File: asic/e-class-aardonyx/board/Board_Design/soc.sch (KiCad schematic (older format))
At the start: 90 parts, among them J1 Conn_01x04, U1 SKT32E, U2 CDCE913PW, Y1 10MHz

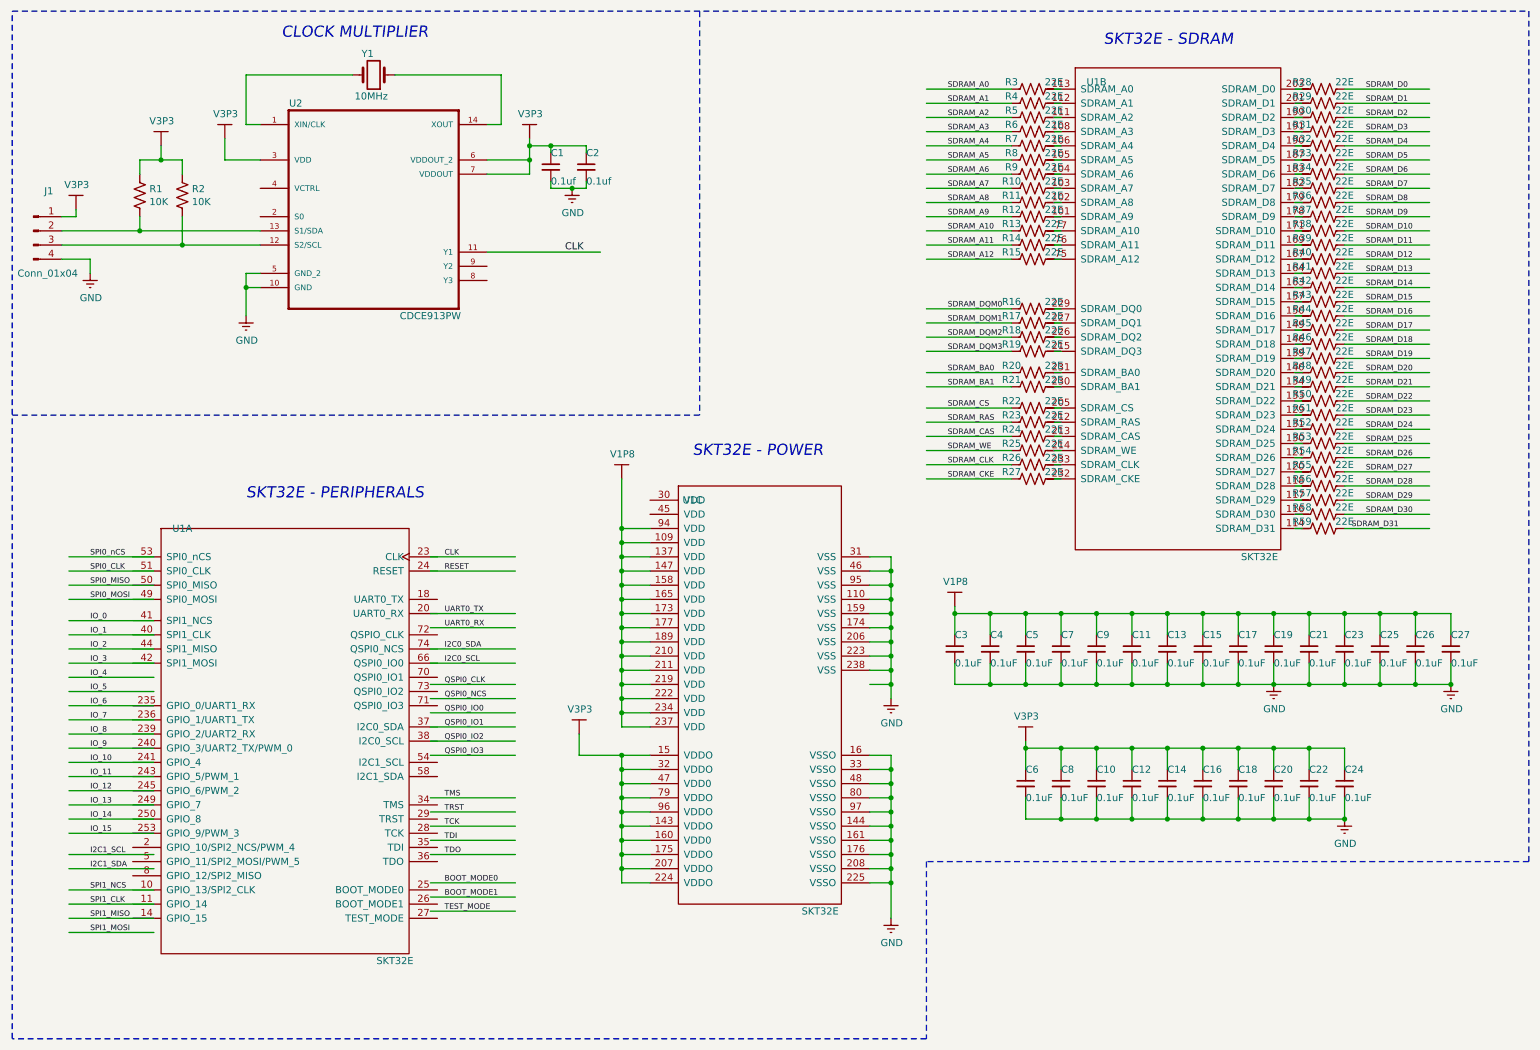
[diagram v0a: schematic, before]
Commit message: update
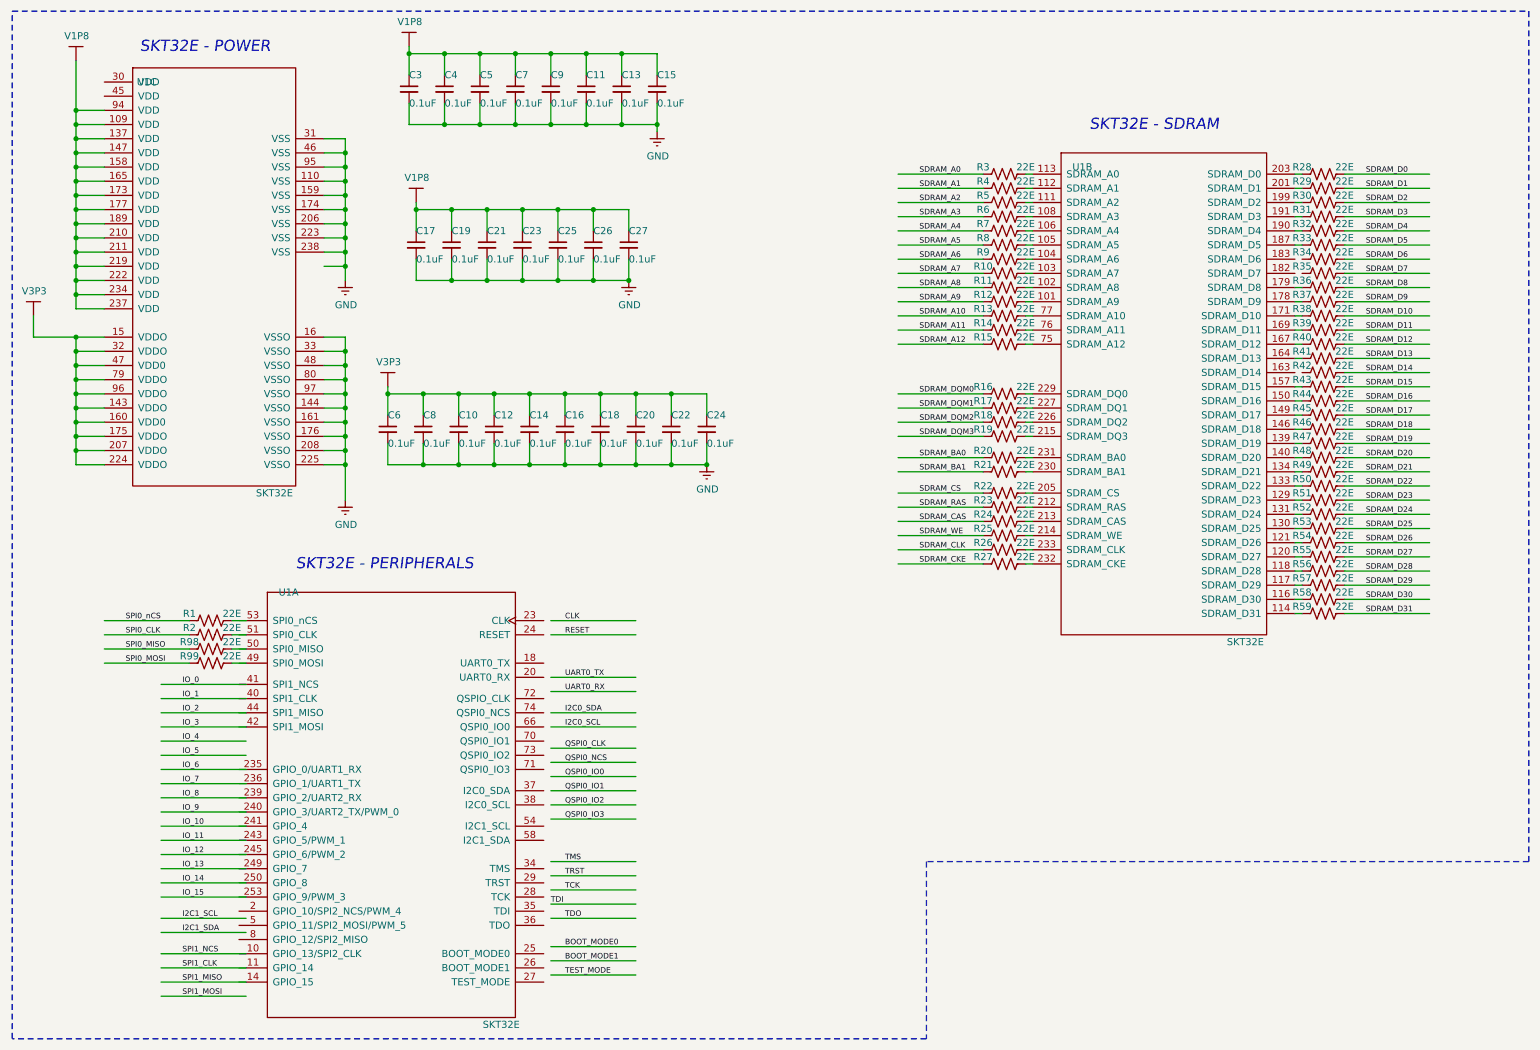
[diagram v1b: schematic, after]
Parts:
- removed C1, C2: 0.1uf, symbol aardonyx:C_Small
- removed J1: Conn_01x04, symbol Connector:Conn_01x04_Male
- removed U2: CDCE913PW, SOP65P640X120-14N, symbol aardonyx:CDCE913PW
- removed Y1: 10MHz, symbol aardonyx:Crystal
- added R98, R99: 22E, symbol aardonyx:R_US
- R1, R2: value 10K -> 22E
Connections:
- wire segments 390 -> 350
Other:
- note removed: "CLOCK MULTIPLIER\n"
- moved on the sheet: C10, C11, C12, C13, C14, C15, C16, C17, C18, C19, C20, C21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

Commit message: update
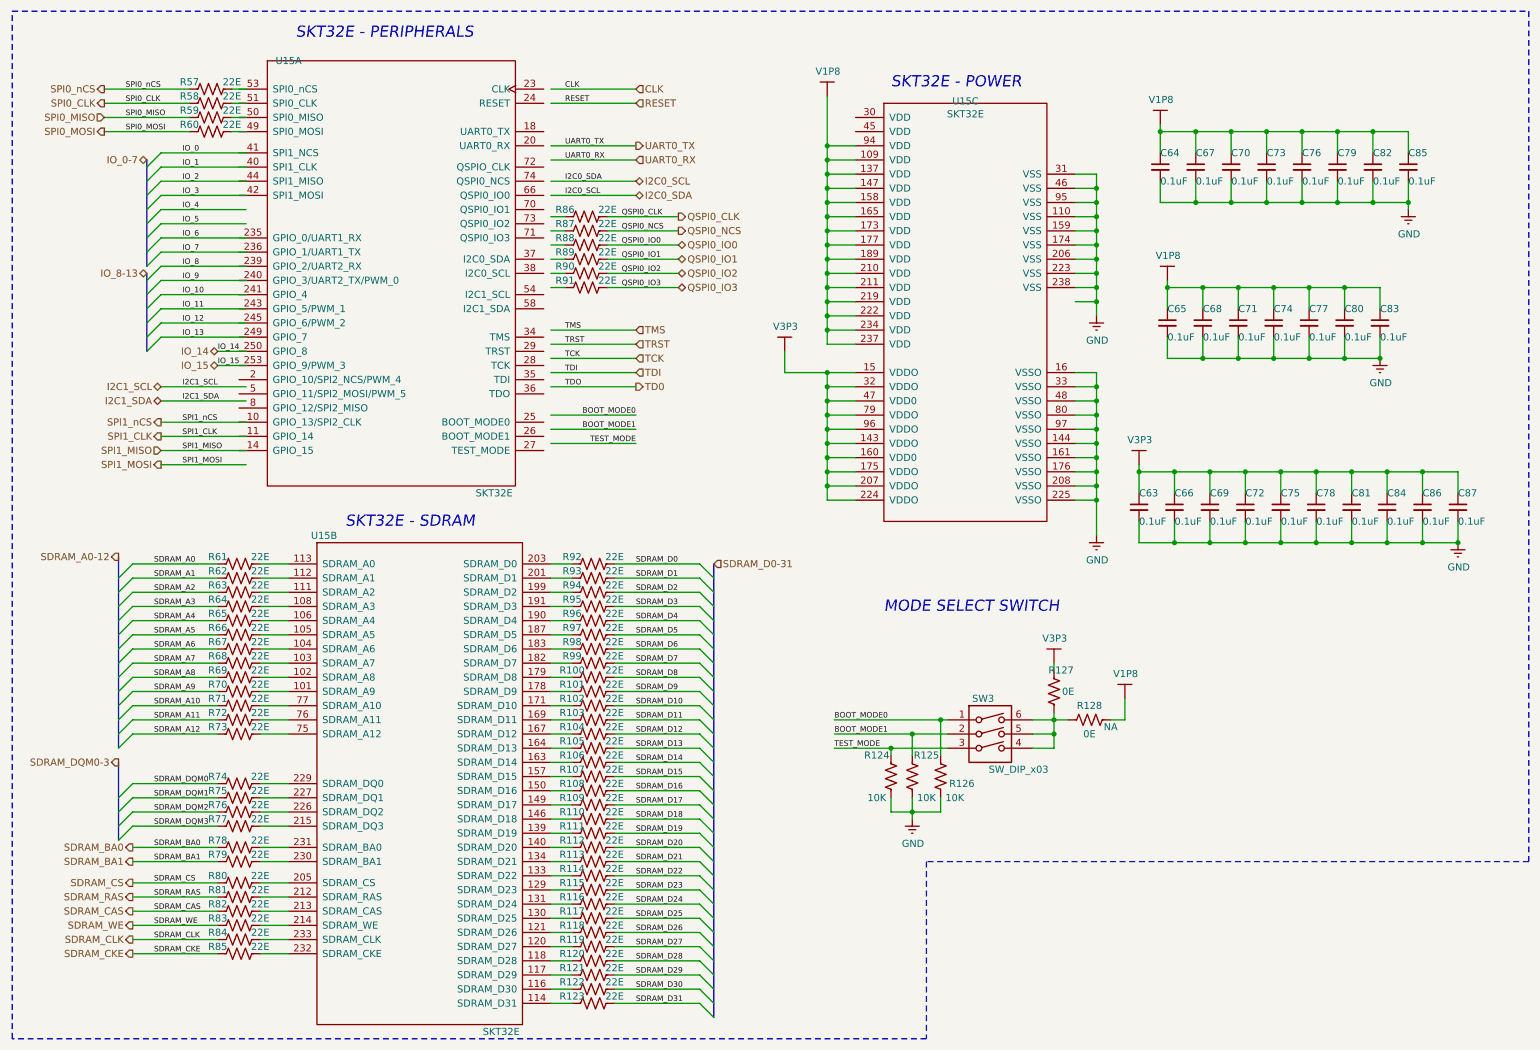
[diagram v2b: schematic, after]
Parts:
- removed U1: SKT32E, symbol aardonyx:SKT32E
- added R124, R125, R126: 10K, symbol aardonyx:R_US
- added R127, R128: 0E, symbol aardonyx:R_US
- added R86, R87, R88, R89, R90, R91: 22E, symbol aardonyx:R_US
- added SW3: SW_DIP_x03, symbol aardonyx:SW_DIP_x03
- added U15: SKT32E, symbol aardonyx:SKT32E
- renumbered C6 to C63, C3 to C64, C17 to C65, C8 to C66, C4 to C67, C19 to C68, C10 to C69, C5 to C70, C21 to C71, C12 to C72, C7 to C73, C23 to C74, C14 to C75, C9 to C76, C25 to C77, C16 to C78, C11 to C79, C26 to C80, C18 to C81, C13 to C82, C27 to C83, C20 to C84, C15 to C85, C22 to C86, C24 to C87, R36 to R100, R37 to R101, R38 to R102, R39 to R103, R40 to R104, R41 to R105, R42 to R106, R43 to R107, R44 to R108, R45 to R109, R46 to R110, R47 to R111, R48 to R112, R49 to R113, R50 to R114, R51 to R115, R52 to R116, R53 to R117, R54 to R118, R55 to R119, R56 to R120, R57 to R121, R58 to R122, R59 to R123, R1 to R57, R2 to R58, R98 to R59, R99 to R60, R3 to R61, R4 to R62, R5 to R63, R6 to R64, R7 to R65, R8 to R66, R9 to R67, R10 to R68, R11 to R69, R12 to R70, R13 to R71, R14 to R72, R15 to R73, R16 to R74, R17 to R75, R18 to R76, R19 to R77, R20 to R78, R21 to R79, R22 to R80, R23 to R81, R24 to R82, R25 to R83, R26 to R84, R27 to R85, R28 to R92, R29 to R93, R30 to R94, R31 to R95, R32 to R96, R33 to R97, R34 to R98, R35 to R99
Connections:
- net labels added: IO_0-7, IO_8-13, SDRAM_A0-12, SDRAM_D0-31, SDRAM_DQM0-3, SPI1_nCS, TD0
- net labels removed: SPI1_NCS
- wire segments 350 -> 384
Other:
- note added: "MODE SELECT SWITCH"
- moved on the sheet: C63, C64, C65, C66, C67, C68, C69, C70, C71, C72, C73, C74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
